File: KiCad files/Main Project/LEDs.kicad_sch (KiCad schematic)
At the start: 4 parts

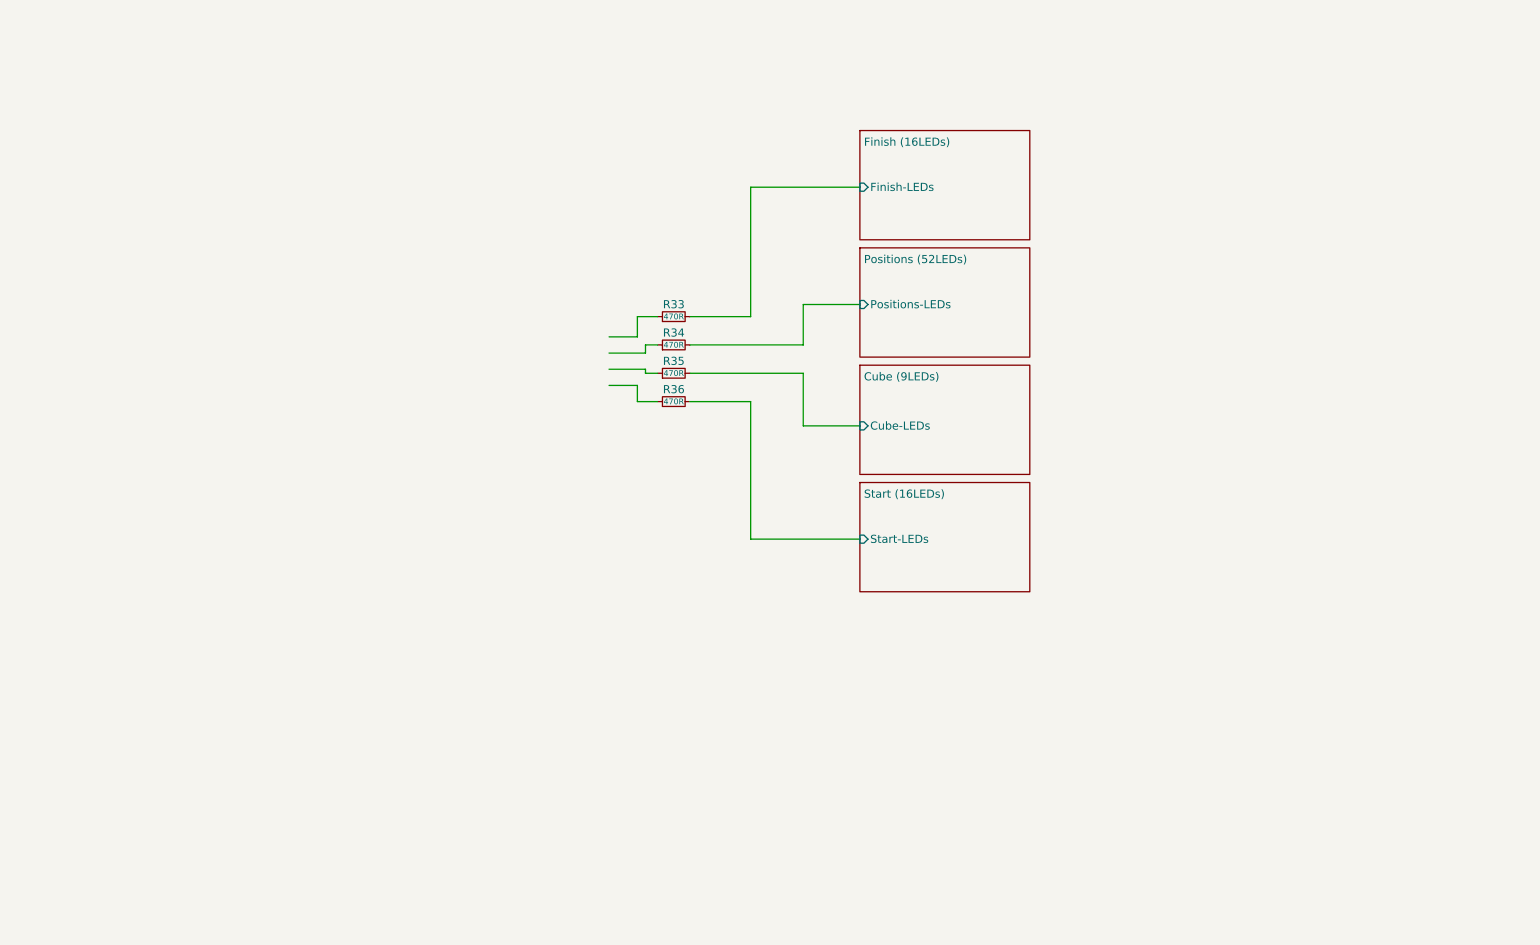
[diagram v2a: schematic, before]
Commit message: update
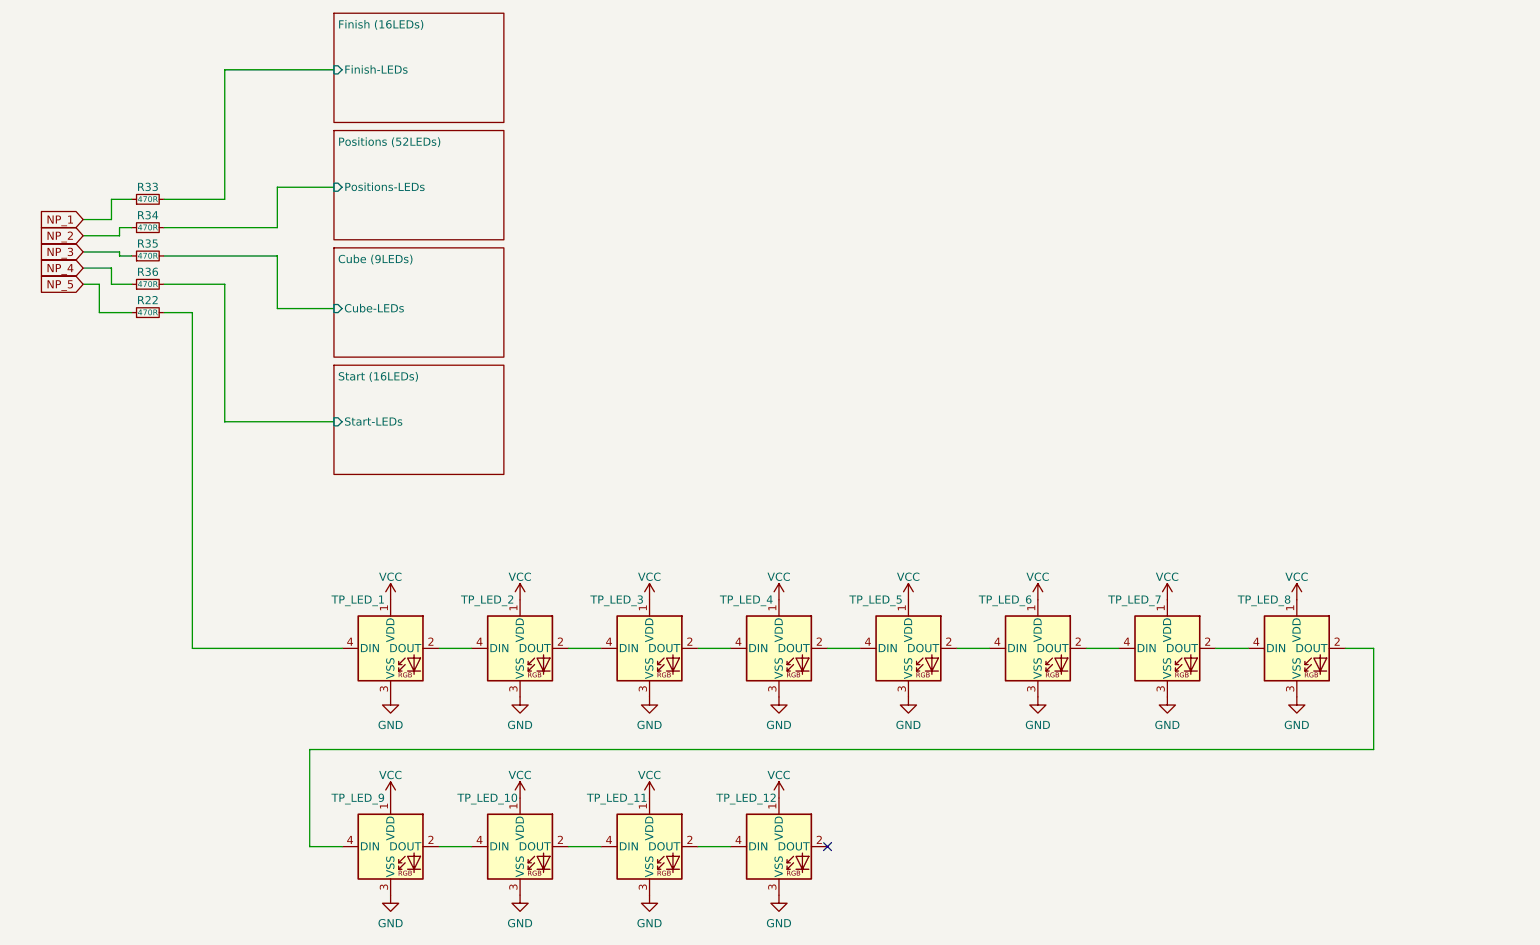
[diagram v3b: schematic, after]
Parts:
- added R22: 470R, Resistor_SMD:R_0603_1608Metric, symbol Device:R_Small
- added TP_LED_1, TP_LED_10, TP_LED_11, TP_LED_12, TP_LED_2, TP_LED_3, TP_LED_4, TP_LED_5, TP_LED_6, TP_LED_7, TP_LED_8, TP_LED_9: WS2812-4020_dual, LED_SMD:LED_WS2812B_PLCC4_5.0x5.0mm_P3.2mm, symbol LED:WS2812B
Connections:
- net NP_2: now reaches R34.1
- net NP_4: now reaches R36.1
- net NP_1: now reaches R33.1
- net NP_3: now reaches R35.1
- new net: TP_LED_8.2 (DOUT), TP_LED_9.4 (DIN)
- new net: TP_LED_7.2 (DOUT), TP_LED_8.4 (DIN)
- new net: TP_LED_3.2 (DOUT), TP_LED_4.4 (DIN)
- new net: TP_LED_2.2 (DOUT), TP_LED_3.4 (DIN)
- new net: TP_LED_11.2 (DOUT), TP_LED_12.4 (DIN)
- new net: TP_LED_10.2 (DOUT), TP_LED_11.4 (DIN)
- new net: TP_LED_1.2 (DOUT), TP_LED_2.4 (DIN)
- new net: R22.2, TP_LED_1.4 (DIN)
- new net: TP_LED_4.2 (DOUT), TP_LED_5.4 (DIN)
- new net: TP_LED_10.4 (DIN), TP_LED_9.2 (DOUT)
- new net: TP_LED_6.2 (DOUT), TP_LED_7.4 (DIN)
- new net: TP_LED_5.2 (DOUT), TP_LED_6.4 (DIN)
- new net GND: TP_LED_1.3 (VSS), TP_LED_10.3 (VSS), TP_LED_11.3 (VSS), TP_LED_12.3 (VSS), TP_LED_2.3 (VSS), TP_LED_3.3 (VSS), TP_LED_4.3 (VSS), TP_LED_5.3 (VSS), TP_LED_6.3 (VSS), TP_LED_7.3 (VSS), TP_LED_8.3 (VSS), TP_LED_9.3 (VSS)
- new net NP_5: R22.1
- new net VCC: TP_LED_1.1 (VDD), TP_LED_10.1 (VDD), TP_LED_11.1 (VDD), TP_LED_12.1 (VDD), TP_LED_2.1 (VDD), TP_LED_3.1 (VDD), TP_LED_4.1 (VDD), TP_LED_5.1 (VDD), TP_LED_6.1 (VDD), TP_LED_7.1 (VDD), TP_LED_8.1 (VDD), TP_LED_9.1 (VDD)
- no-connect marks 0 -> 1
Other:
- moved on the sheet: R33, R34, R35, R36

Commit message: shematic update
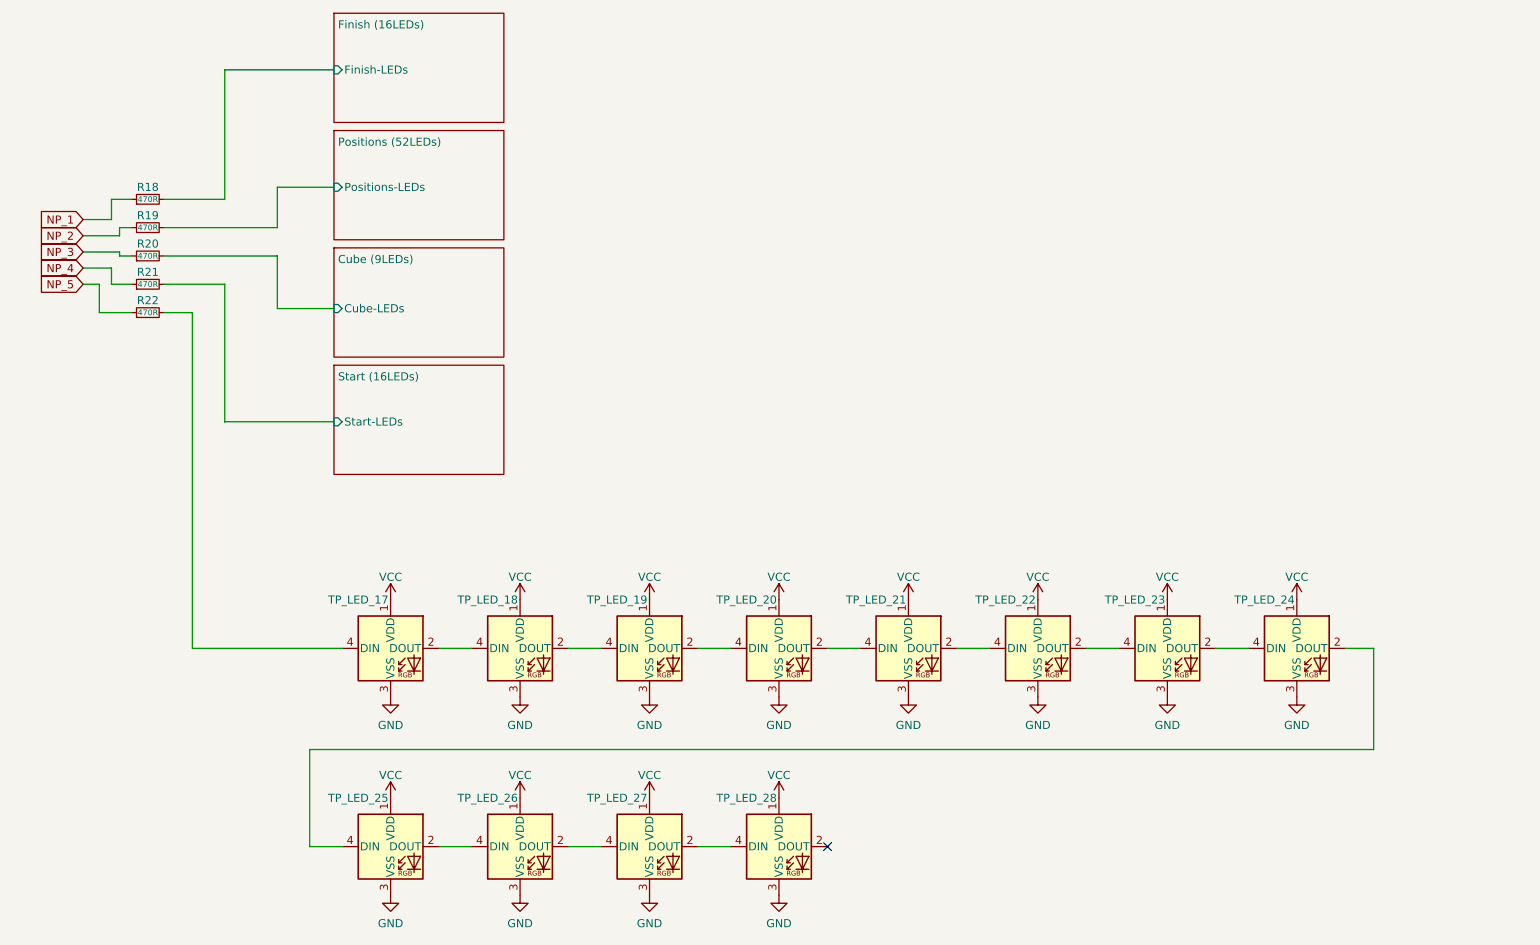
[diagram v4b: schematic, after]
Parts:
- renumbered R33 to R18, R34 to R19, R35 to R20, R36 to R21, TP_LED_1 to TP_LED_17, TP_LED_2 to TP_LED_18, TP_LED_3 to TP_LED_19, TP_LED_4 to TP_LED_20, TP_LED_5 to TP_LED_21, TP_LED_6 to TP_LED_22, TP_LED_7 to TP_LED_23, TP_LED_8 to TP_LED_24, TP_LED_9 to TP_LED_25, TP_LED_10 to TP_LED_26, TP_LED_11 to TP_LED_27, TP_LED_12 to TP_LED_28

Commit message: update
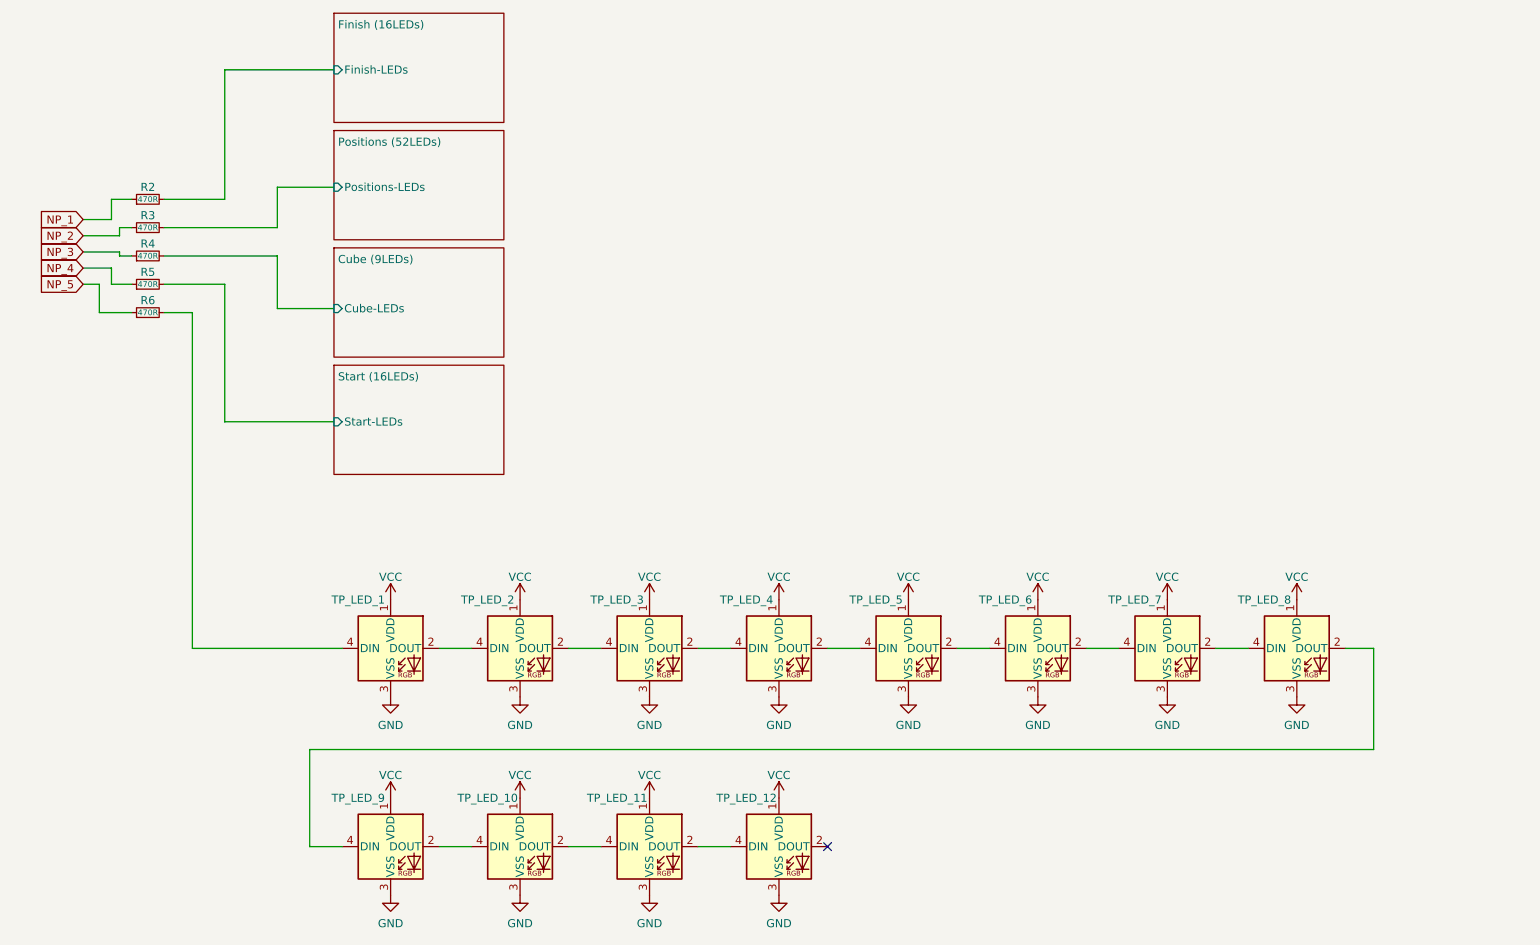
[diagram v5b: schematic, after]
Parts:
- renumbered R18 to R2, R19 to R3, R20 to R4, R21 to R5, R22 to R6, TP_LED_17 to TP_LED_1, TP_LED_26 to TP_LED_10, TP_LED_27 to TP_LED_11, TP_LED_28 to TP_LED_12, TP_LED_18 to TP_LED_2, TP_LED_19 to TP_LED_3, TP_LED_20 to TP_LED_4, TP_LED_21 to TP_LED_5, TP_LED_22 to TP_LED_6, TP_LED_23 to TP_LED_7, TP_LED_24 to TP_LED_8, TP_LED_25 to TP_LED_9
